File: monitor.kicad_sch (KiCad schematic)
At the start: 50 parts, among them J1 Conn_01x01_Socket, J2 Conn_01x01_Socket, J3 Conn_01x01_Socket, J4 Conn_01x01_Socket, J5 Conn_01x01_Socket, J6 Conn_01x01_Socket, U704 OPA2197D, U71 TMUX6104, U72 TMUX6104, U76 OPA2189DGK, U77 OPA2388DGK, U78 OPA2189DGK

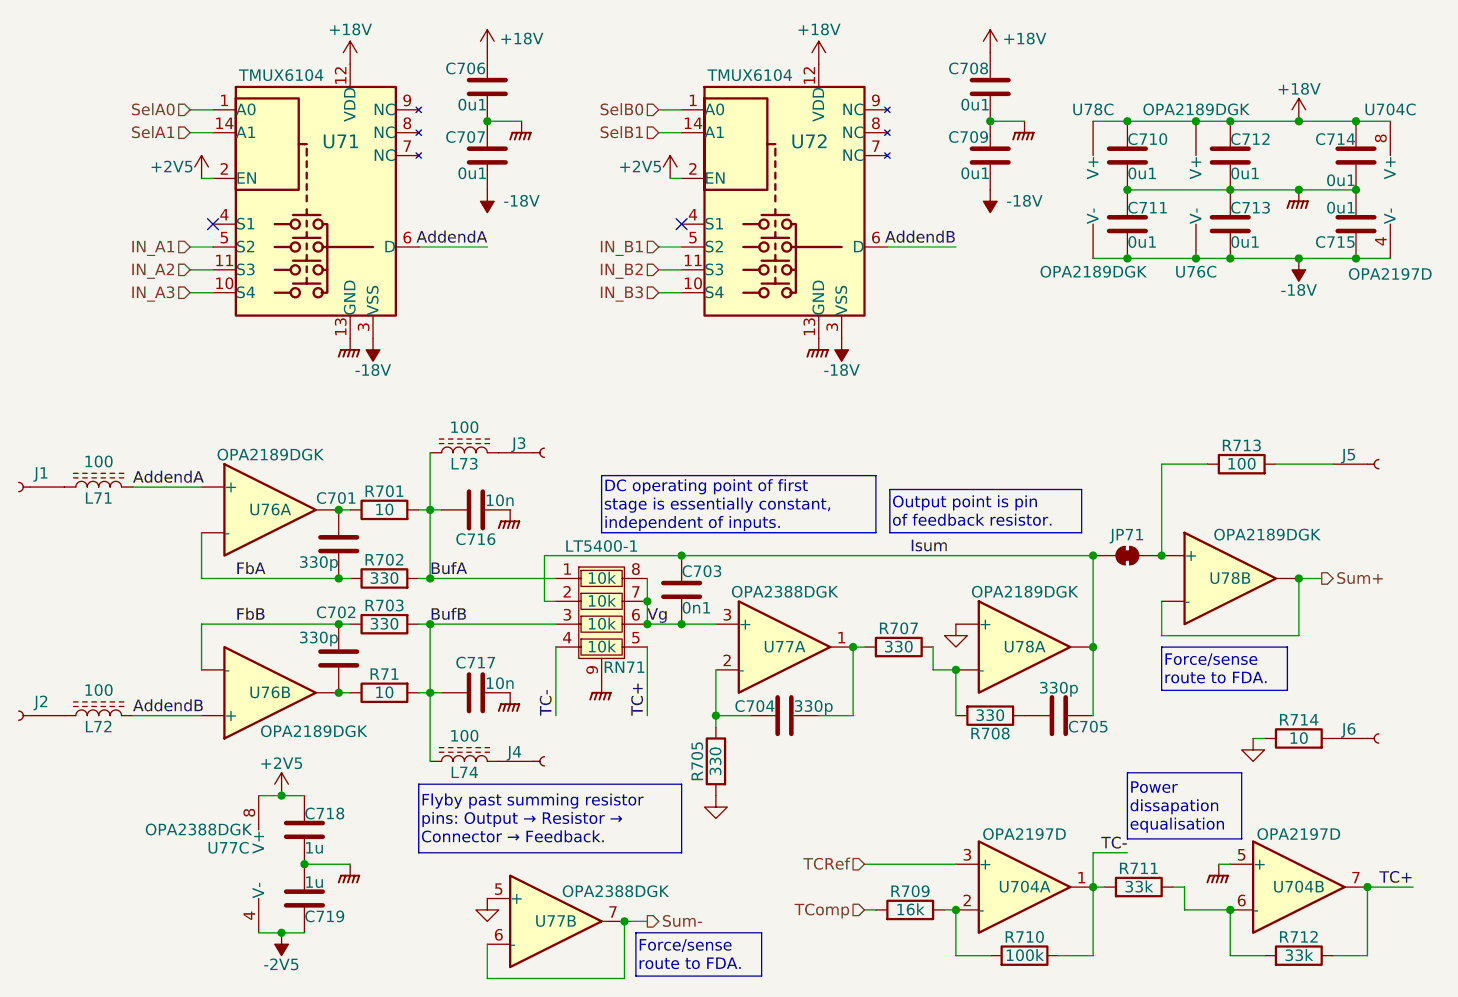
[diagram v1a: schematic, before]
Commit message: Most blocks there....
About to restore scan.
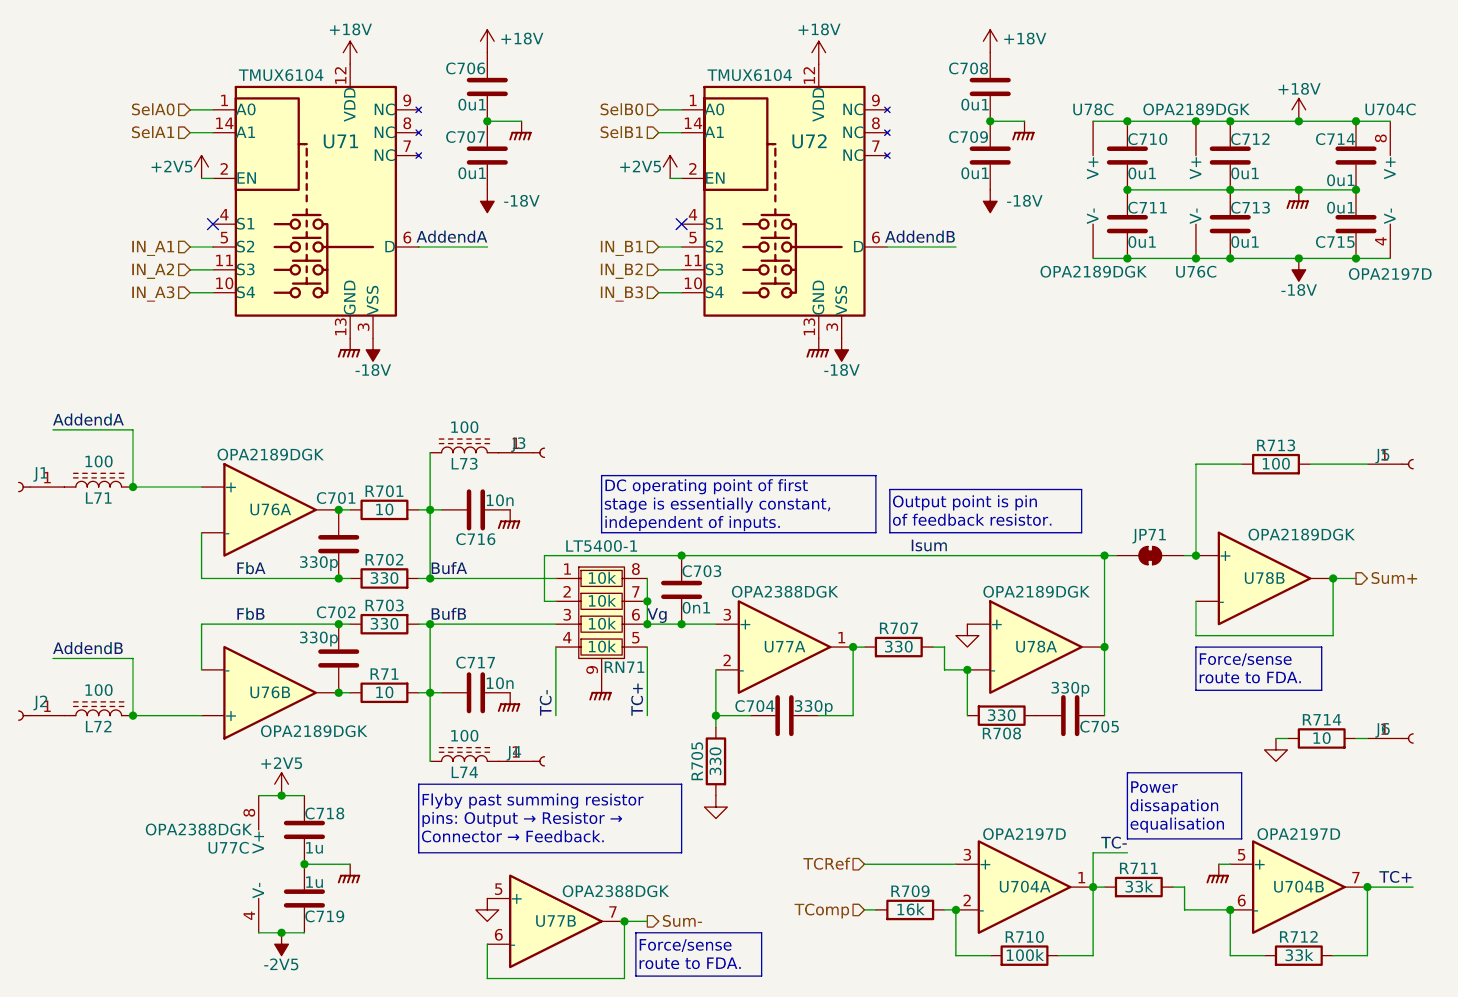
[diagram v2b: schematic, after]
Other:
- moved on the sheet: C705, JP71, R708, R713, R714, U78A, U78B
